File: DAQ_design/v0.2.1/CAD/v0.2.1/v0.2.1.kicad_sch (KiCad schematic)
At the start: 2 parts, among them U1 Teensy4.0, U2 TLV6001DCK

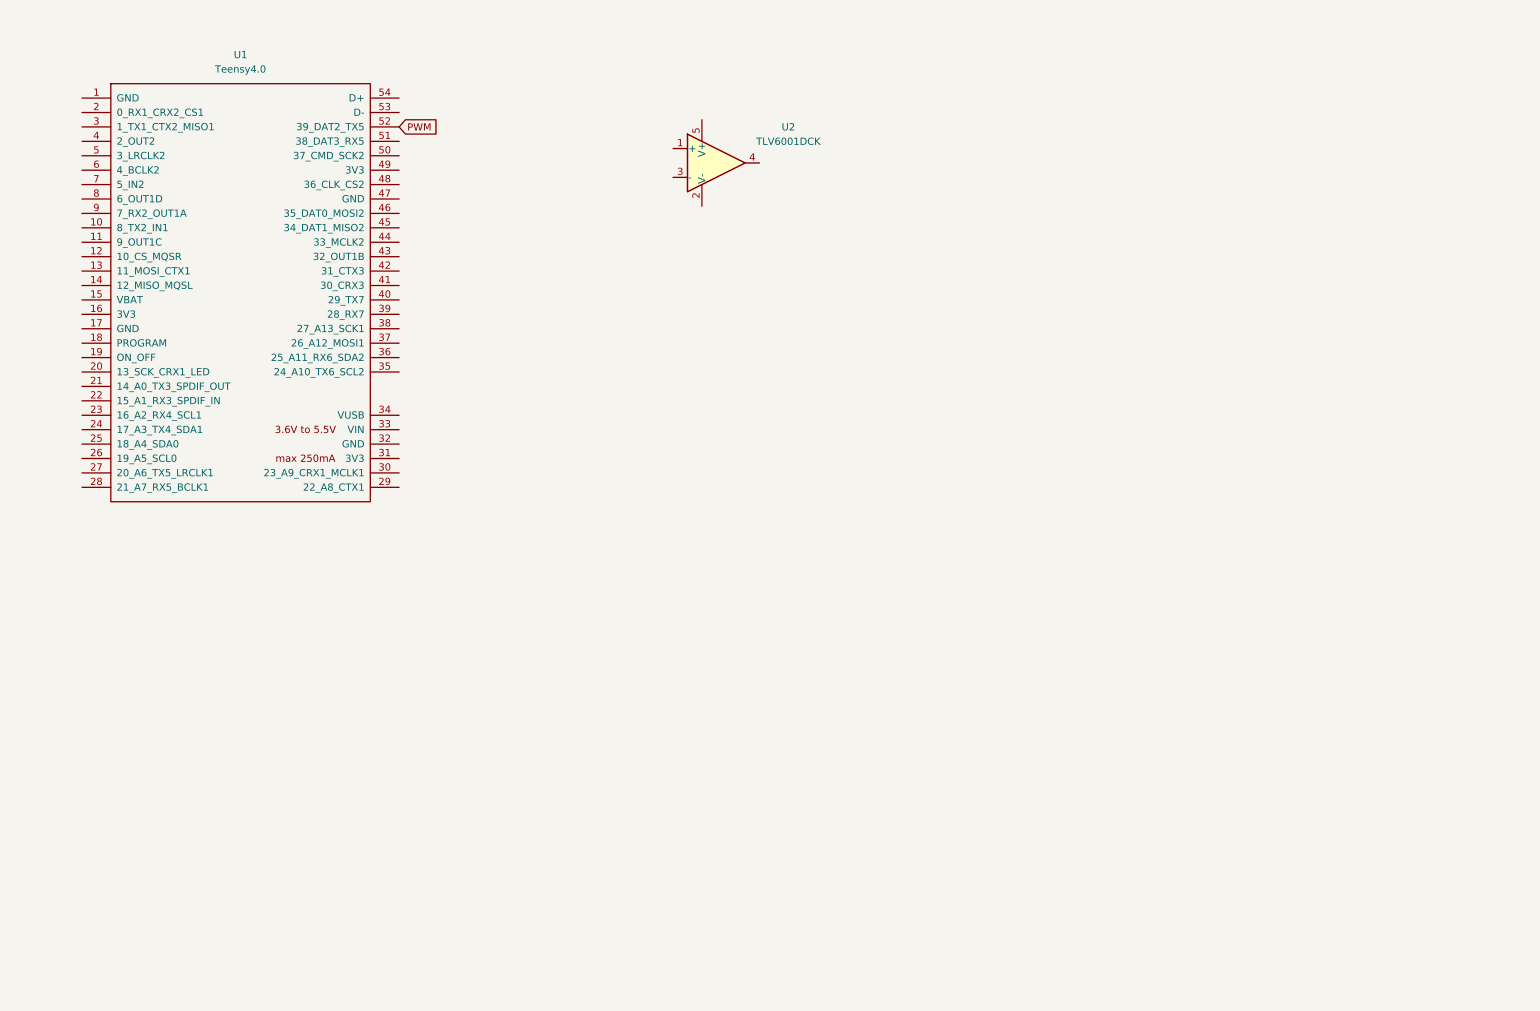
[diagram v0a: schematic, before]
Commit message: new code and cad
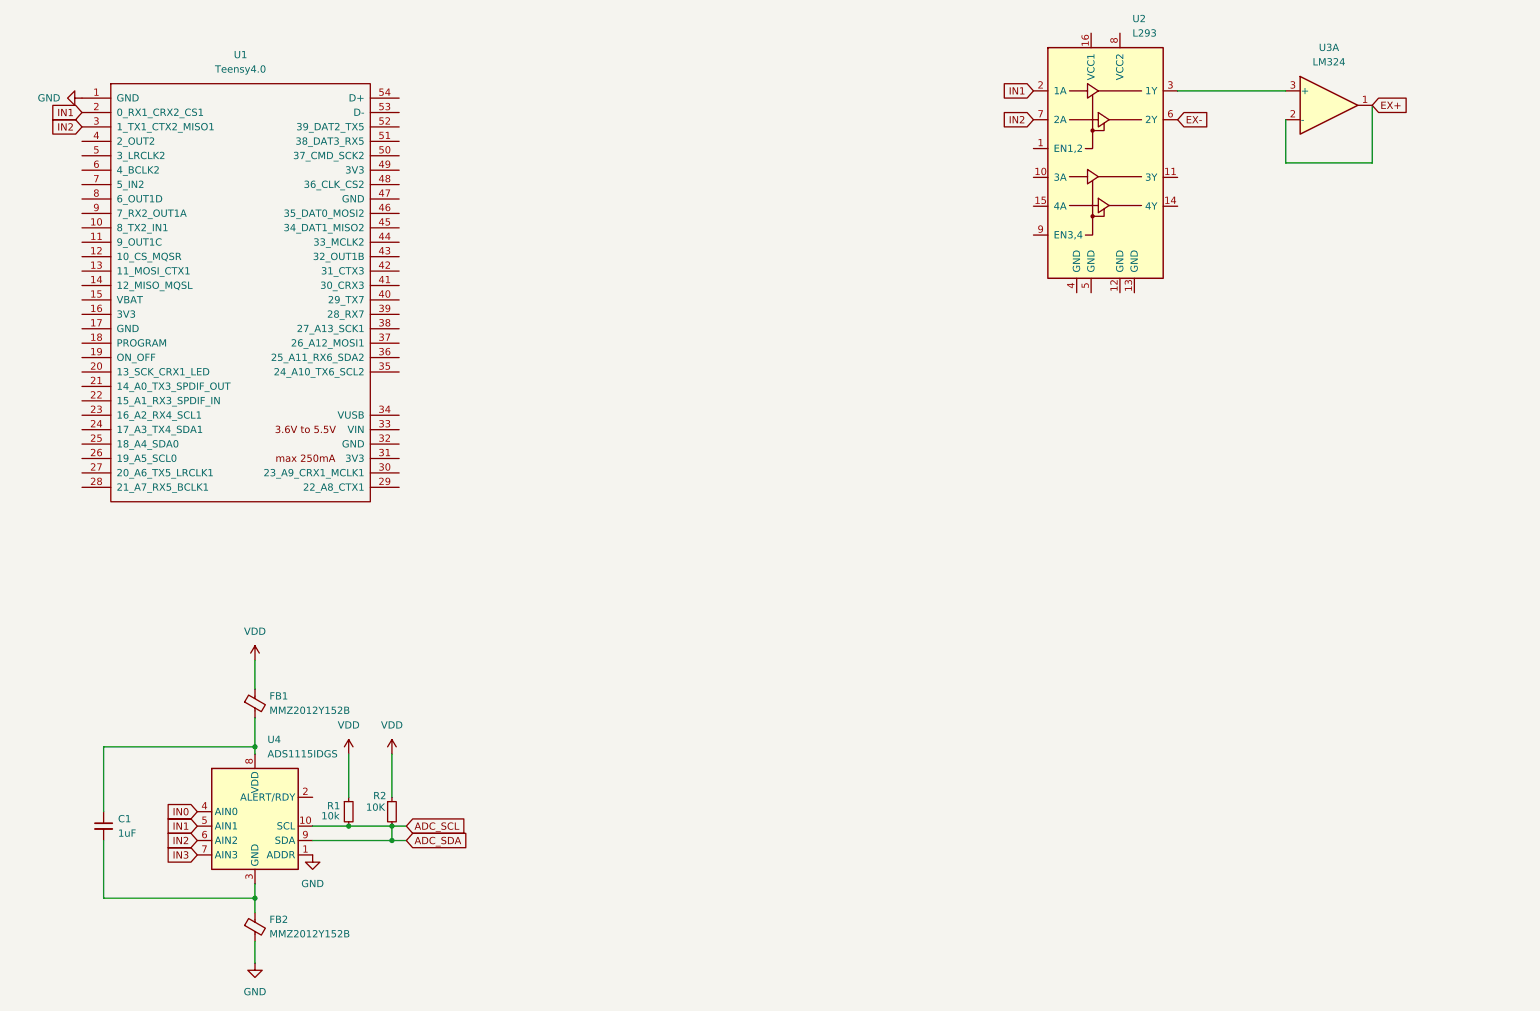
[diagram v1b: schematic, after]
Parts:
- removed U2: TLV6001DCK, Package_TO_SOT_SMD:SOT-353_SC-70-5, symbol Amplifier_Operational:TLV6001DCK
- added C1: 1uF, symbol Device:C_Small
- added FB1, FB2: MMZ2012Y152B, symbol Device:FerriteBead_Small
- added R1: 10k, symbol Device:R_Small
- added R2: 10K, symbol Device:R_Small
- added U2: L293, Package_DIP:DIP-16_W7.62mm, symbol Driver_Motor:L293
- added U3: LM324, symbol Amplifier_Operational:LM324
- added U4: ADS1115IDGS, Package_SO:TSSOP-10_3x3mm_P0.5mm, symbol Analog_ADC:ADS1115IDGS
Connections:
- net GND: now reaches U1.1 (GND)
- net GND: now also FB2.2, U4.1 (ADDR)
- net IN1: now reaches U1.2 (0_RX1_CRX2_CS1)
- net IN1: now also U2.2 (1A), U4.5 (AIN1)
- net IN2: now reaches U1.3 (1_TX1_CTX2_MISO1)
- net IN2: now also U2.7 (2A), U4.6 (AIN2)
- net PWM: no longer names the net of U1.52 (39_DAT2_TX5)
- new net: C1.2, FB2.1, U4.3 (GND)
- new net: U2.3 (1Y), U3.3 (+)
- new net: C1.1, FB1.2, U4.8 (VDD)
- new net ADC_SCL: R1.2, R2.2, U4.10 (SCL), U4.9 (SDA)
- new net EX+: U3.1, U3.2 (-)
- new net EX-: U2.6 (2Y)
- new net IN0: U4.4 (AIN0)
- new net IN3: U4.7 (AIN3)
- new net VDD: FB1.1, R1.1, R2.1

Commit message: pushing test figures
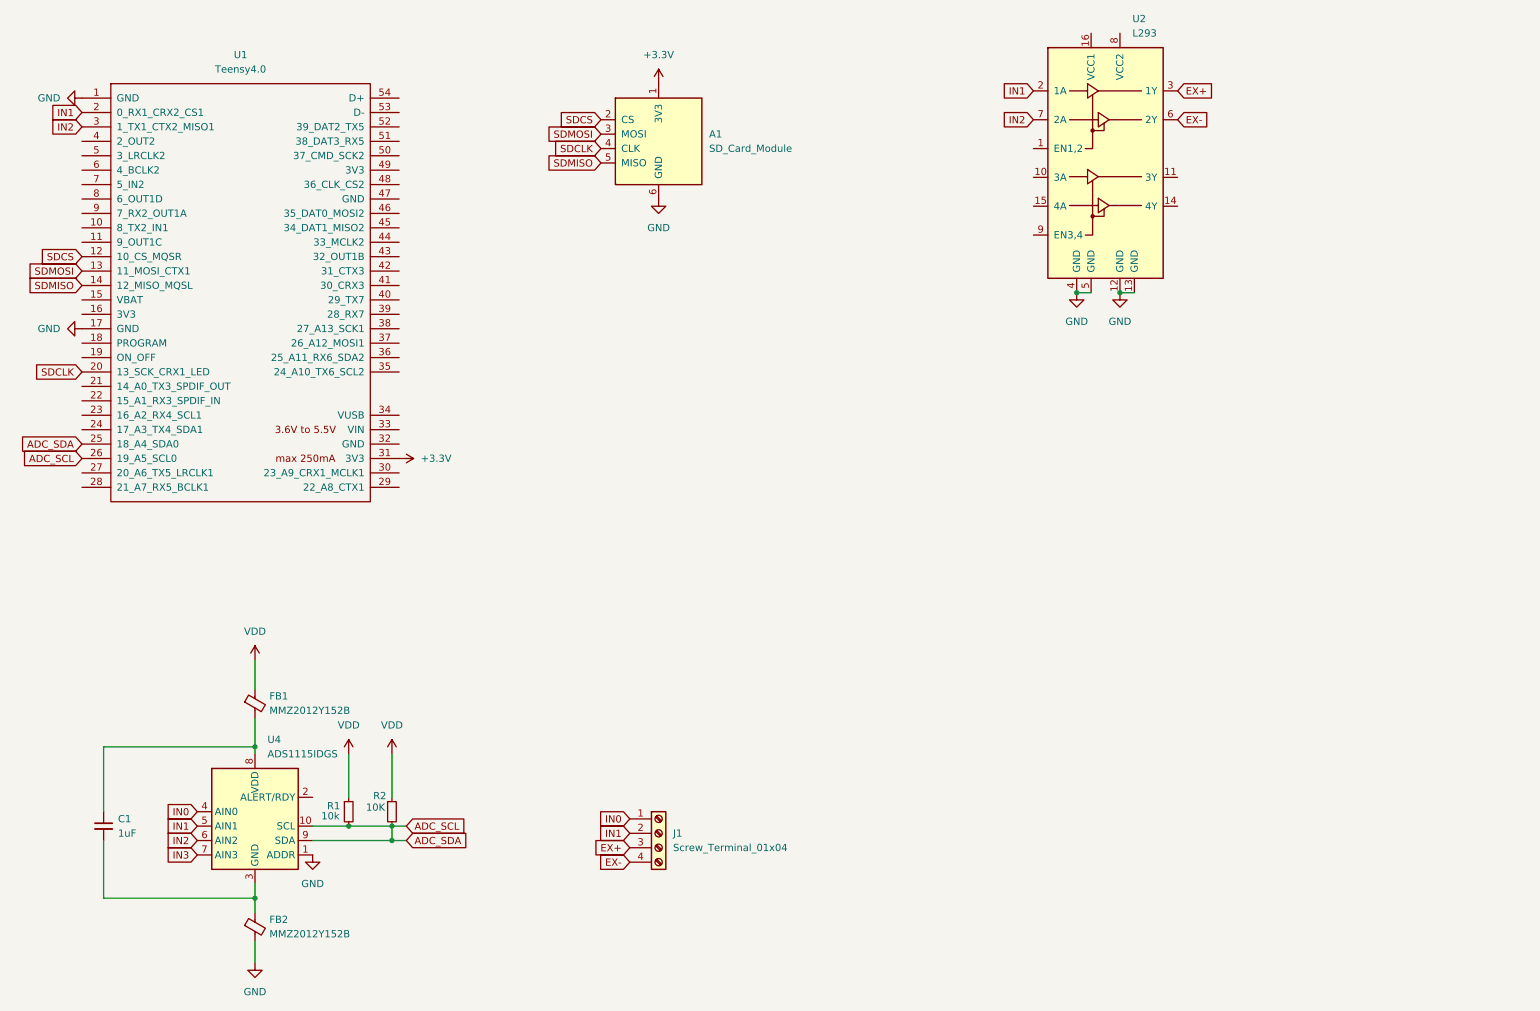
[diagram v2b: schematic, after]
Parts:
- removed U3: LM324, symbol Amplifier_Operational:LM324
- added A1: SD_Card_Module, Charleslabs_Parts:SD_Card_Module, symbol Charleslabs_Parts:SD_Card_Module
- added J1: Screw_Terminal_01x04, symbol Connector:Screw_Terminal_01x04
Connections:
- net ADC_SCL: now also U1.25 (18_A4_SDA0), U1.26 (19_A5_SCL0)
- net EX+: now also U2.3 (1Y), J1.3 (Pin_3)
- net EX-: now also J1.4 (Pin_4)
- net GND: now also U1.17 (GND), U2.12 (GND), U2.13 (GND), U2.4 (GND), U2.5 (GND), A1.6 (GND)
- net IN0: now also J1.1 (Pin_1)
- net IN1: now also J1.2 (Pin_2)
- net SDCS: now reaches U1.12 (10_CS_MQSR)
- net SDCS: now also A1.2 (CS)
- net SDMOSI: now reaches U1.13 (11_MOSI_CTX1)
- net SDMOSI: now also A1.3 (MOSI)
- net SDMISO: now reaches U1.14 (12_MISO_MQSL)
- net SDMISO: now also A1.5 (MISO)
- net SDCLK: now reaches U1.20 (13_SCK_CRX1_LED)
- net SDCLK: now also A1.4 (CLK)
- net +3.3V: now reaches U1.31 (3V3)
- net +3.3V: now also A1.1 (3V3)

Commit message: tests and cad
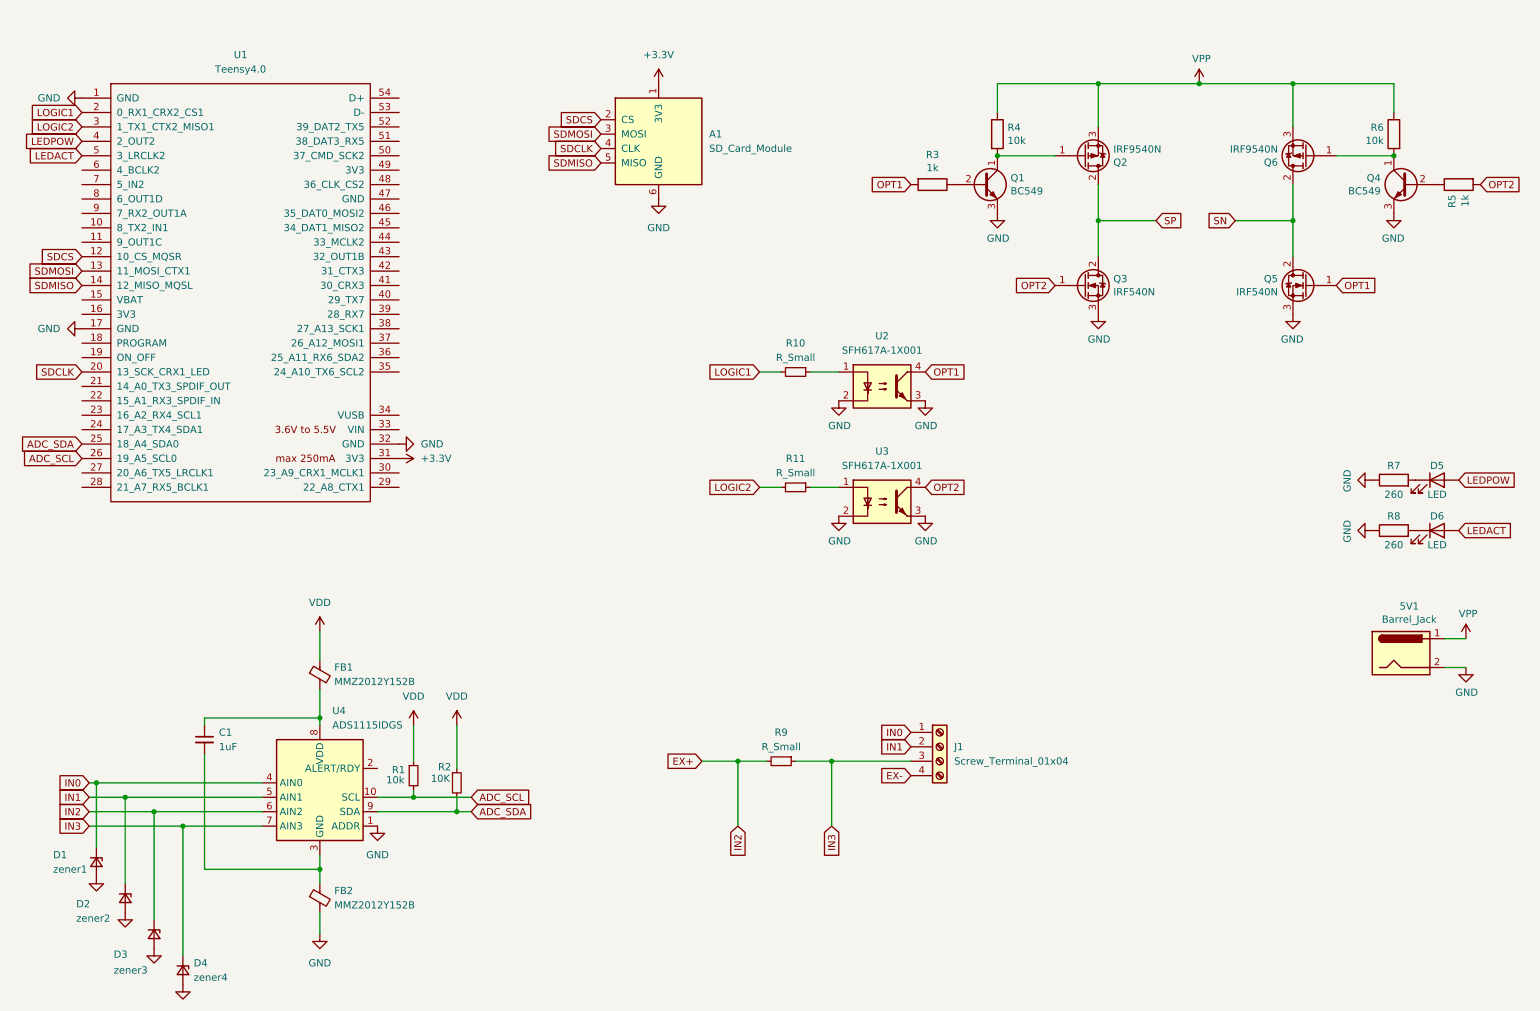
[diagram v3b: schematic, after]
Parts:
- removed U2: L293, Package_DIP:DIP-16_W7.62mm, symbol Driver_Motor:L293
- added 5V1: Barrel_Jack, Connector_BarrelJack:BarrelJack_Horizontal, symbol Connector:Barrel_Jack
- added D1: zener1, Diode_SMD:D_1206_3216Metric, symbol Device:D_Zener_Small
- added D2: zener2, Diode_SMD:D_1206_3216Metric, symbol Device:D_Zener_Small
- added D3: zener3, Diode_SMD:D_1206_3216Metric, symbol Device:D_Zener_Small
- added D4: zener4, Diode_SMD:D_1206_3216Metric, symbol Device:D_Zener_Small
- added D5, D6: LED, LED_SMD:LED_1206_3216Metric, symbol Device:LED
- added Q1, Q4: BC549, Package_TO_SOT_THT:TO-92_Inline_Wide, symbol Transistor_BJT:BC549
- added Q2, Q6: IRF9540N, Package_TO_SOT_THT:TO-220-3_Vertical, symbol Transistor_FET:IRF9540N
- added Q3, Q5: IRF540N, Package_TO_SOT_THT:TO-220-3_Vertical, symbol Transistor_FET:IRF540N
- added R10, R11, R9: R_Small, Resistor_SMD:R_1206_3216Metric, symbol Device:R_Small
- added R3, R5: 1k, Resistor_SMD:R_1206_3216Metric, symbol Device:R
- added R4, R6: 10k, Resistor_SMD:R_1206_3216Metric, symbol Device:R
- added R7, R8: 260, Resistor_SMD:R_1206_3216Metric, symbol Device:R
- added U2, U3: SFH617A-1X001, Package_DIP:DIP-4_W7.62mm, symbol Isolator:SFH617A-1X001
- C1: footprint (none) -> Capacitor_SMD:C_1206_3216Metric
- FB1, FB2: footprint (none) -> Inductor_SMD:L_Ferrocore_DLG-0302
- J1: footprint (none) -> TerminalBlock:TerminalBlock_bornier-4_P5.08mm
- R1, R2: footprint (none) -> Resistor_SMD:R_1206_3216Metric
- U1: footprint (none) -> teensy.pretty-master:Teensy40
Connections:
- net ADC_SCL: no longer R2.2, U1.25 (18_A4_SDA0), U4.9 (SDA)
- net EX+: now also U4.6 (AIN2), D3.1 (K), R9.2; no longer J1.3 (Pin_3)
- net GND: now also U1.32 (GND), 5V1.2, D1.2 (A), D2.2 (A), D3.2 (A), D4.2 (A), Q1.3 (E), Q3.3 (S), Q4.3 (E), Q5.3 (S), R7.1, R8.1, U2.2, U2.3, U3.2, U3.3
- net IN0: now also D1.1 (K)
- net IN1: now also D2.1 (K); no longer U1.2 (0_RX1_CRX2_CS1)
- net IN3: now also J1.3 (Pin_3), D4.1 (K), R9.1
- net LEDPOW: now reaches U1.4 (2_OUT2)
- net LEDPOW: now also D5.2 (A)
- net LEDACT: now reaches U1.5 (3_LRCLK2)
- net LEDACT: now also D6.2 (A)
- net IN2 renamed LOGIC2
- net LOGIC2: now also R11.2; no longer U4.6 (AIN2)
- new net: Q4.1 (C), Q6.1 (G), R6.2
- new net: R10.1, U2.1
- new net: Q1.1 (C), Q2.1 (G), R4.2
- new net: Q1.2 (B), R3.1
- new net: D5.1 (K), R7.2
- new net: R11.1, U3.1
- new net: Q4.2 (B), R5.1
- new net: D6.1 (K), R8.2
- new net ADC_SDA: R2.2, U1.25 (18_A4_SDA0), U4.9 (SDA)
- new net LOGIC1: R10.2, U1.2 (0_RX1_CRX2_CS1)
- new net OPT1: Q5.1 (G), R3.2, U2.4
- new net OPT2: Q3.1 (G), R5.2, U3.4
- new net SN: Q5.2 (D), Q6.2 (D)
- new net SP: Q2.2 (D), Q3.2 (D)
- new net VPP: 5V1.1, Q2.3 (S), Q6.3 (S), R4.1, R6.1
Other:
- moved on the sheet: C1, FB1, FB2, J1, R1, R2, U4
